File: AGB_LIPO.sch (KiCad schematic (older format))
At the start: 11 parts, among them J1 Conn_01x02_Male, Q1 Si2301DS, U1 misc_tp4056_board-tp4056, U2 AMS1117-3.3

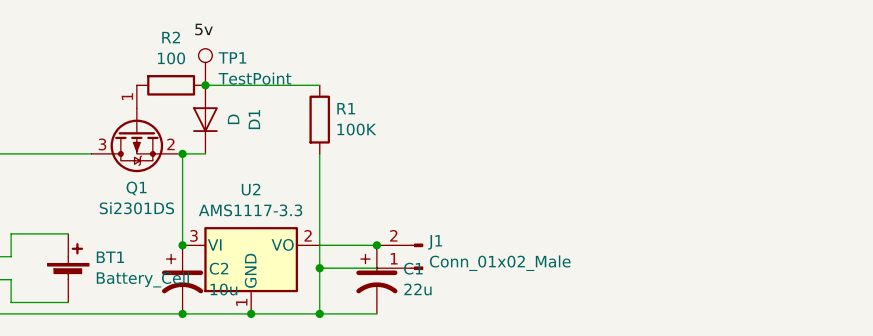
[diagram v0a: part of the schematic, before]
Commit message: Full Circuit redesign
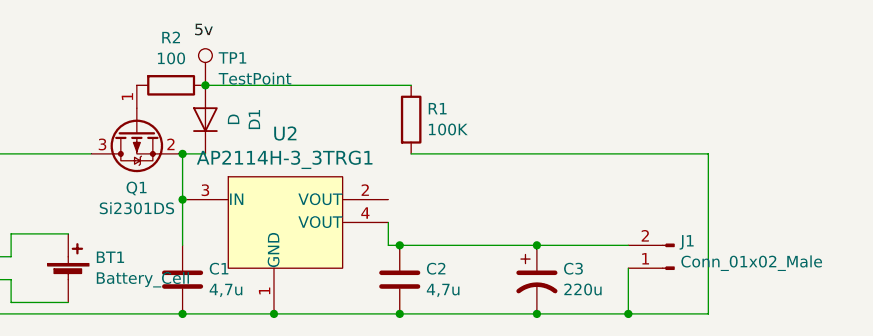
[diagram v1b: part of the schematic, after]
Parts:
- removed C1: 22u, Capacitor_Tantalum_SMD:CP_EIA-3216-18_Kemet-A, symbol Device:CP1
- removed C2: 10u, Capacitor_Tantalum_SMD:CP_EIA-3216-18_Kemet-A, symbol Device:CP1
- removed U2: AMS1117-3.3, Package_TO_SOT_SMD:SOT-223-3_TabPin2, symbol Regulator_Linear:AMS1117-3.3
- added C1, C2: 4,7u, Capacitor_SMD:C_0603_1608Metric, symbol Device:C
- added C3: 220u, Capacitor_Tantalum_SMD:CP_EIA-3528-21_Kemet-B, symbol Device:CP1
- added U2: AP2114H-3_3TRG1, digikey-footprints:SOT-223, symbol Libraries_digikey-kicad-library-master_digikey-symbols_dk_PMIC-Voltage-Regulato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
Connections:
- net at J1.1 (Pin_1), R1.2, U1.6 (GND_OUT): now also C1.2, C2.2, C3.2, U2.1 (GND)
- net at J1.2 (Pin_2): now also C2.1, C3.1, U2.4 (VOUT)
- net at D1.1 (K), Q1.2 (S): now also C1.1, U2.3 (IN)
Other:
- moved on the sheet: J1, R1
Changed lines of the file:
@@
-$EndComp
-$Comp
-L Device:R R1
-U 1 1 5EA0FDCF
-P 6700 2800
-F 0 "R1" H 6770 2846 50  0000 L CNN
-F 1 "100K" H 6770 2755 50  0000 L CNN
-F 2 "Resistor_THT:R_Axial_DIN0204_L3.6mm_D1.6mm_P7.62mm_Horizontal" V 6630 2800 50  0001 C CNN
-F 3 "~" H 6700 2800 50  0001 C CNN
-	1    6700 2800
-	1    0    0    -1
 $EndComp
 $Comp
@@
 	5600 3300 5350 3300
 $Comp
-L Connector:Conn_01x02_Male J1
-U 1 1 5E2E1CEE
-P 7150 3450
-F 0 "J1" H 7122 3332 50  0000 R CNN
-F 1 "Conn_01x02_Male" H 7122 3423 50  0000 R CNN
-F 2 "TestPoint:TestPoint_2Pads_Pitch2.54mm_Drill0.8mm" H 7150 3450 50  0001 C CNN
-F 3 "~" H 7150 3450 50  0001 C CNN
-	1    7150 3450
-	-1   0    0    1
-$EndComp
-$Comp
 L Device:Battery_Cell BT1
 U 1 1 5E2E12D0
@@
 	1    0    0    -1
 $EndComp
+Text Label 6150 2450 0    50   ~ 0
+5v
+Wire Wire Line
+	5250 2950 5700 2950
+Wire Wire Line
+	6100 2950 6100 3150
+$Comp
+L Device:R R2
+U 1 1 5EA6A02A
+P 6050 2650
+F 0 "R2" V 5843 2650 50  0000 C CNN
+F 1 "100" V 5934 2650 50  0000 C CNN
+F 2 "Resistor_THT:R_Axial_DIN0204_L3.6mm_D1.6mm_P7.62mm_Horizontal" V 5980 2650 50  0001 C CNN
+F 3 "~" H 6050 2650 50  0001 C CNN
+	1    6050 2650
+	0    1    1    0
+$EndComp
+Connection ~ 6200 2650
 $Comp
 L Device:D D1
@@
 $EndComp
 $Comp
-L Regulator_Linear:AMS1117-3.3 U2
-U 1 1 5EA50985
-P 6400 3350
-F 0 "U2" H 6400 3592 50  0000 C CNN
-F 1 "AMS1117-3.3" H 6400 3501 50  0000 C CNN
-F 2 "Package_TO_SOT_SMD:SOT-223-3_TabPin2" H 6400 3550 50  0001 C CNN
-F 3 "http://www.advanced-monolithic.com/pdf/ds1117.pdf" H 6500 3100 50  0001 C CNN
-	1    6400 3350
+L Connector:Conn_01x02_Male J1
+U 1 1 5E2E1CEE
+P 8250 3450
+F 0 "J1" H 8222 3332 50  0000 R CNN
+F 1 "Conn_01x02_Male" H 8222 3423 50  0000 R CNN
+F 2 "TestPoint:TestPoint_2Pads_Pitch2.54mm_Drill0.8mm" H 8250 3450 50  0001 C CNN
+F 3 "~" H 8250 3450 50  0001 C CNN
+	1    8250 3450
+	-1   0    0    1
+$EndComp
+$Comp
+L Device:R R1
+U 1 1 5EA0FDCF
+P 7100 2800
+F 0 "R1" H 7170 2846 50  0000 L CNN
+F 1 "100K" H 7170 2755 50  0000 L CNN
+F 2 "Resistor_THT:R_Axial_DIN0204_L3.6mm_D1.6mm_P7.62mm_Horizontal" V 7030 2800 50  0001 C CNN
+F 3 "~" H 7100 2800 50  0001 C CNN
+	1    7100 2800
 	1    0    0    -1
 $EndComp
-Wire Wire Line
-	6400 3650 6700 3650
-Wire Wire Line
-	6700 3450 6700 3650
-Wire Wire Line
-	5250 3650 6100 3650
-Connection ~ 6400 3650
-Text Label 6150 2450 0    50   ~ 0
-5v
-Wire Wire Line
-	5250 2950 5700 2950
-Wire Wire Line
-	6100 2950 6100 3350
-$Comp
-L Device:R R2
-U 1 1 5EA6A02A
-P 6050 2650
-F 0 "R2" V 5843 2650 50  0000 C CNN
-F 1 "100" V 5934 2650 50  0000 C CNN
-F 2 "Resistor_THT:R_Axial_DIN0204_L3.6mm_D1.6mm_P7.62mm_Horizontal" V 5980 2650 50  0001 C CNN
-F 3 "~" H 6050 2650 50  0001 C CNN
-	1    6050 2650
-	0    1    1    0
-$EndComp
-Connection ~ 6200 2650
+Connection ~ 6100 2950
 Wire Wire Line
 	6100 2950 6200 2950
-Connection ~ 6100 2950
+$Comp
+L Libraries_digikey-kicad-library-master_digikey-symbols_dk_PMIC-Voltage-Regulators-Linear:AP2114H-3_3TRG1 U2
+U 1 1 5EABEFBA
+P 6600 3150
+F 0 "U2" H 6550 3437 60  0000 C CNN
+F 1 "AP2114H-3_3TRG1" H 6550 3331 60  0000 C CNN
+F 2 "digikey-footprints:SOT-223" H 6800 3350 60  0001 L CNN
+F 3 "https://www.diodes.com/assets/Datasheets/AP2114.pdf" H 6800 3450 60  0001 L CNN
+F 4 "AP2114H-3.3TRG1DICT-ND" H 6800 3550 60  0001 L CNN "Digi-Key_PN"
+F 5 "AP2114H-3.3TRG1" H 6800 3650 60  0001 L CNN "MPN"
+F 6 "Integrated Circuits (ICs)" H 6800 3750 60  0001 L CNN "Category"
+F 7 "PMIC - Voltage Regulators - Linear" H 6800 3850 60  0001 L CNN "Family"
+F 8 "https://www.diodes.com/assets/Datasheets/AP2114.pdf" H 6800 3950 60  0001 L CNN "DK_Datasheet_Link"
+F 9 "/product-detail/en/diodes-incorporated/AP2114H-3.3TRG1/AP2114H-3.3TRG1DICT-ND/4505142" H 6800 4050 60  0001 L CNN "DK_Detail_Page"
+F 10 "IC REG LINEAR 3.3V 1A SOT223" H 6800 4150 60  0001 L CNN "Description"
+F 11 "Diodes Incorporated" H 6800 4250 60  0001 L CNN "Manufacturer"
+F 12 "Active" H 6800 4350 60  0001 L CNN "Status"
+	1    6600 3150
+	1    0    0    -1
+$EndComp
+Connection ~ 6500 3650
 Wire Wire Line
-	6700 3650 6950 3650
-Connection ~ 6700 3650
+	6500 3650 7050 3650
+Connection ~ 6100 3150
 Wire Wire Line
-	6700 3450 6950 3450
-Wire Wire Line
-	6200 2650 6700 2650
-Wire Wire Line
-	6950 3350 6700 3350
-Connection ~ 6100 3350
-Connection ~ 6100 3650
-Wire Wire Line
-	6100 3650 6400 3650
-Connection ~ 6700 3450
-Wire Wire Line
-	6700 2950 6700 3450
+	6100 3150 6100 3350
 $Comp
-L Device:CP1 C2
-U 1 1 5EA9F1F5
+L Device:C C1
+U 1 1 5EAC7AF3
 P 6100 3500
-F 0 "C2" H 6215 3546 50  0000 L CNN
-F 1 "10u" H 6215 3455 50  0000 L CNN
-F 2 "Capacitor_Tantalum_SMD:CP_EIA-3216-18_Kemet-A" H 6100 3500 50  0001 C CNN
+F 0 "C1" H 6215 3546 50  0000 L CNN
+F 1 "4,7u" H 6215 3455 50  0000 L CNN
+F 2 "Capacitor_SMD:C_0603_1608Metric" H 6100 3500 50  0001 C CNN
 F 3 "~" H 6100 3500 50  0001 C CNN
 	1    6100 3500
 	1    0    0    -1
 $EndComp
+Connection ~ 6100 3650
+Wire Wire Line
+	6100 3650 6500 3650
 $Comp
-L Device:CP1 C1
-U 1 1 5EAA0031
-P 6950 3500
-F 0 "C1" H 7065 3546 50  0000 L CNN
-F 1 "22u" H 7065 3455 50  0000 L CNN
-F 2 "Capacitor_Tantalum_SMD:CP_EIA-3216-18_Kemet-A" H 6950 3500 50  0001 C CNN
-F 3 "~" H 6950 3500 50  0001 C CNN
-	1    6950 3500
+L Device:C C2
+U 1 1 5EAC7F3D
+P 7050 3500
+F 0 "C2" H 7165 3546 50  0000 L CNN
+F 1 "4,7u" H 7165 3455 50  0000 L CNN
+F 2 "Capacitor_SMD:C_0603_1608Metric" H 7050 3500 50  0001 C CNN
+F 3 "~" H 7050 3500 50  0001 C CNN
+	1    7050 3500
 	1    0    0    -1
 $EndComp
-Connection ~ 6950 3350
+Connection ~ 7050 3650
+Wire Wire Line
+	7000 3250 7000 3350
+Wire Wire Line
+	7000 3350 7050 3350
+Wire Wire Line
+	6200 2650 7100 2650
+Wire Wire Line
+	5250 3650 6100 3650
+Wire Wire Line
+	7050 3650 7650 3650
+Wire Wire Line
+	7050 3350 7650 3350
+Connection ~ 7050 3350
+Wire Wire Line
+	8050 3450 8050 3650
+Wire Wire Line
+	8050 3650 8400 3650
+Wire Wire Line
+	8400 3650 8400 2950
+Wire Wire Line
+	7100 2950 8400 2950
+Connection ~ 8050 3650
+$Comp
+L Device:CP1 C3
+U 1 1 5EAD4F6D
+P 7650 3500
+F 0 "C3" H 7765 3546 50  0000 L CNN
+F 1 "220u" H 7765 3455 50  0000 L CNN
+F 2 "Capacitor_Tantalum_SMD:CP_EIA-3528-21_Kemet-B" H 7650 3500 50  0001 C CNN
+F 3 "~" H 7650 3500 50  0001 C CNN
+	1    7650 3500
+	1    0    0    -1
+$EndComp
+Connection ~ 7650 3350
+Wire Wire Line
+	7650 3350 8050 3350
+Connection ~ 7650 3650
+Wire Wire Line
+	7650 3650 8050 3650
 $EndSCHEMATC

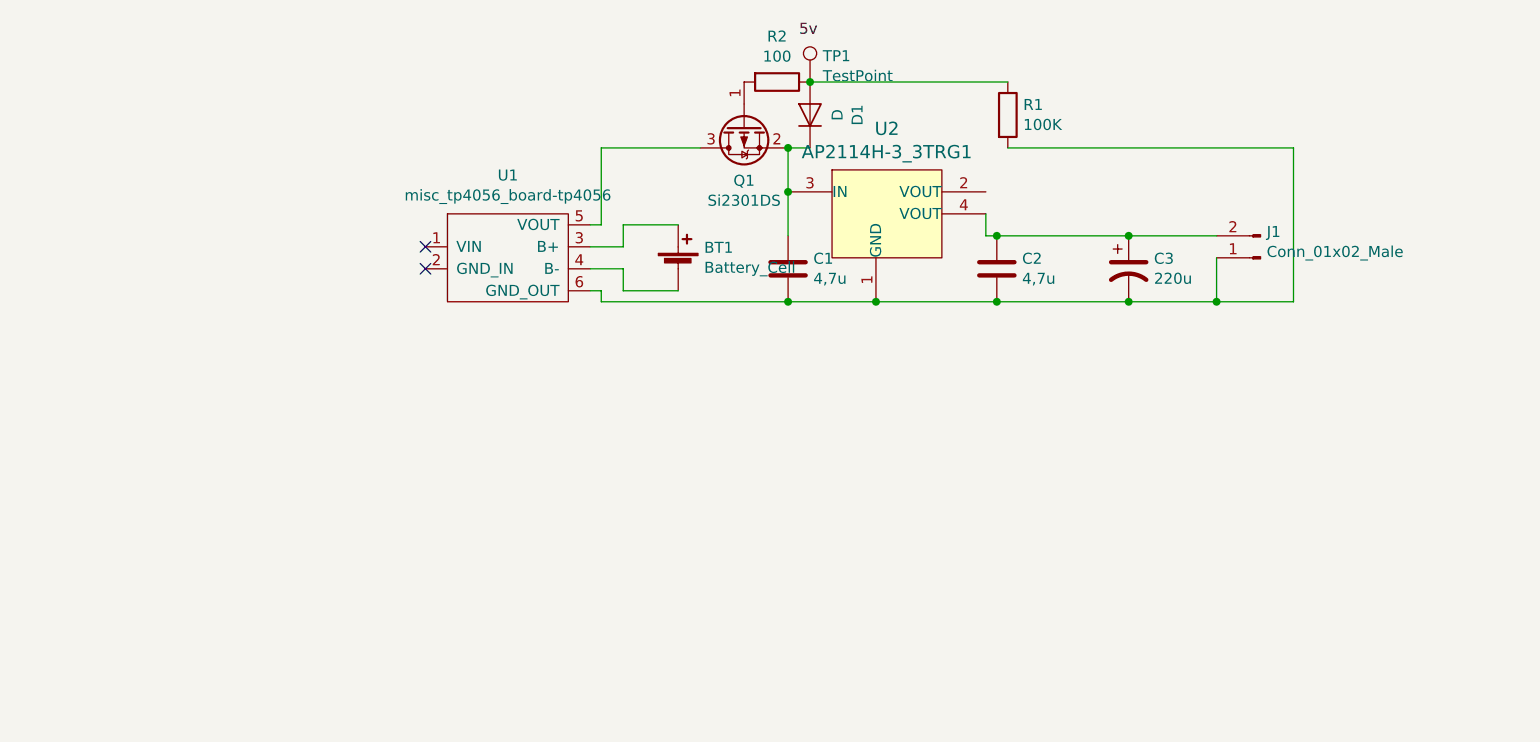
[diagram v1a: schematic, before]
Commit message: 17.06 UPDATE
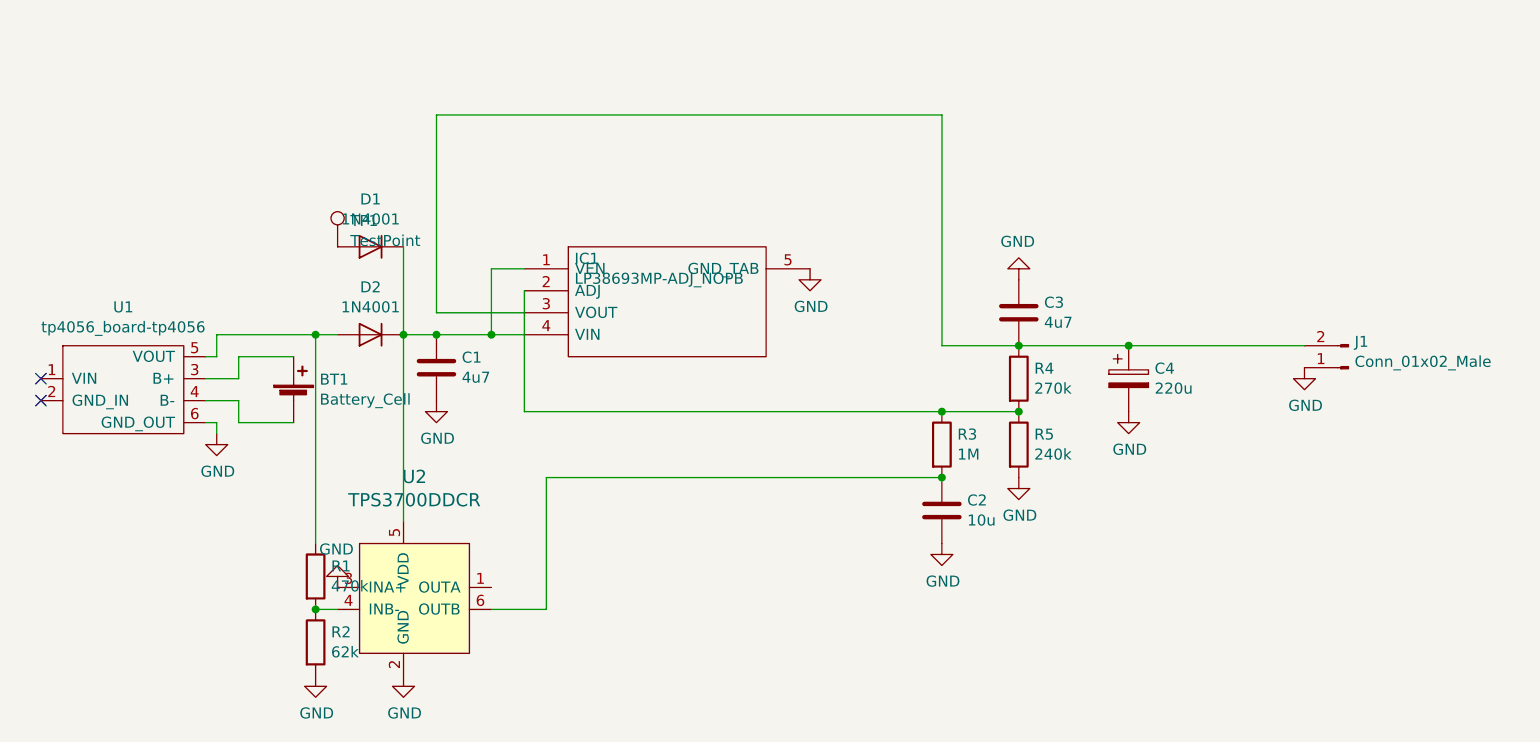
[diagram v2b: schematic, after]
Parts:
- removed C3: 220u, Capacitor_Tantalum_SMD:CP_EIA-3528-21_Kemet-B, symbol Device:CP1
- removed Q1: Si2301DS, Package_TO_SOT_SMD:SOT-23, symbol Transistor_FET:Si2319CDS
- removed U2: AP2114H-3_3TRG1, digikey-footprints:SOT-223, symbol Libraries_digikey-kicad-library-master_digikey-symbols_dk_PMIC-Voltage-Regulato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
- added C3: 4u7, Capacitor_SMD:C_0603_1608Metric_Pad1.05x0.95mm_HandSolder, symbol Device:C
- added C4: 220u, Capacitor_Tantalum_SMD:CP_EIA-3528-21_Kemet-B_Pad1.50x2.35mm_HandSolder, symbol Device:CP
- added D2: 1N4001, SamacSys_Parts:DIOM5626X245N, symbol Device:D
- added IC1: LP38693MP-ADJ_NOPB, SamacSys_Parts:SOT150P700X180-5N, symbol SamacSys_Parts:LP38693MP-ADJ_NOPB
- added R3: 1M, Resistor_SMD:R_0603_1608Metric_Pad1.05x0.95mm_HandSolder, symbol Device:R
- added R4: 270k, Resistor_SMD:R_0805_2012Metric_Pad1.15x1.40mm_HandSolder, symbol Device:R
- added R5: 240k, Resistor_SMD:R_0805_2012Metric_Pad1.15x1.40mm_HandSolder, symbol Device:R
- added U2: TPS3700DDCR, SamacSys_Parts:SOT98P280X110-6N, symbol Libraries_digikey-kicad-library-master_digikey-symbols_dk_Linear-Comparators:TP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
- C1: value 4,7u -> 4u7; footprint Capacitor_SMD:C_0603_1608Metric -> Capacitor_SMD:C_0603_1608Metric_Pad1.05x0.95mm_HandSolder
- C2: value 4,7u -> 10u; footprint Capacitor_SMD:C_0603_1608Metric -> Capacitor_SMD:C_0603_1608Metric_Pad1.05x0.95mm_HandSolder
- D1: value D -> 1N4001; footprint Diode_THT:D_DO-34_SOD68_P7.62mm_Horizontal -> SamacSys_Parts:DIOM5626X245N
- R1: value 100K -> 470k; footprint Resistor_THT:R_Axial_DIN0204_L3.6mm_D1.6mm_P7.62mm_Horizontal -> Resistor_SMD:R_0603_1608Metric_Pad1.05x0.95mm_HandSolder
- R2: value 100 -> 62k; footprint Resistor_THT:R_Axial_DIN0204_L3.6mm_D1.6mm_P7.62mm_Horizontal -> Resistor_SMD:R_0805_2012Metric_Pad1.15x1.40mm_HandSolder
- TP1: footprint TestPoint:TestPoint_THTPad_D1.0mm_Drill0.5mm -> TestPoint:TestPoint_Loop_D1.80mm_Drill1.0mm_Beaded
- U1: value misc_tp4056_board-tp4056 -> tp4056_board-tp4056; footprint kiCad_mod:TP4056-18650 -> digikey-footprints:4056E_LiIon_loader
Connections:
- net GND: now reaches C1.2, C2.2, J1.1 (Pin_1), U1.6 (GND_OUT)
- net GND: now also R2.2, C3.1, C4.2, IC1.5 (GND_TAB), R5.2, U2.2 (GND), U2.3 (INA+); no longer R1.2
- net at J1.2 (Pin_2): now also C3.2, C4.1, IC1.3 (VOUT), R4.1; no longer C2.1
- net at U1.5 (VOUT): now also R1.1, D2.2 (A)
- net at C1.1, D1.1 (K): now also D2.1 (K), IC1.1 (VEN), IC1.4 (VIN), U2.5 (VDD)
- net at D1.2 (A), TP1.1: no longer R1.1, R2.1
- new net: R1.2, R2.1, U2.4 (INB-)
- new net: C2.1, R3.2, U2.6 (OUTB)
- new net: IC1.2 (ADJ), R3.1, R4.2, R5.1
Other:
- moved on the sheet: BT1, J1
